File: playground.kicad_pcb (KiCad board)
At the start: 2 copper layers, 80 x 80 mm, 75 parts, among them IC1 TXU0101DBVR, IC11 LM3940IMP-3.3_NOPB, IC2 TXU0101DBVR, IC3 TXU0101DBVR, IC4 TXU0101DBVR, IC5 TXU0101DBVR, IC6 TXU0101DBVR, IC7 TXU0101DBVR, IC8 TXU0101DBVR, IC9 L293DD, J1 67643-2910, J2 Pump, J3 Fan, J4 Valve, J5 Conn_02x05_Counter_Clockwise, J6 MOLEX POWER CONNECTOR, SW1 SW_DIP_x01, U2 ATSAMD21G18A-A, Y1 32.768kHz

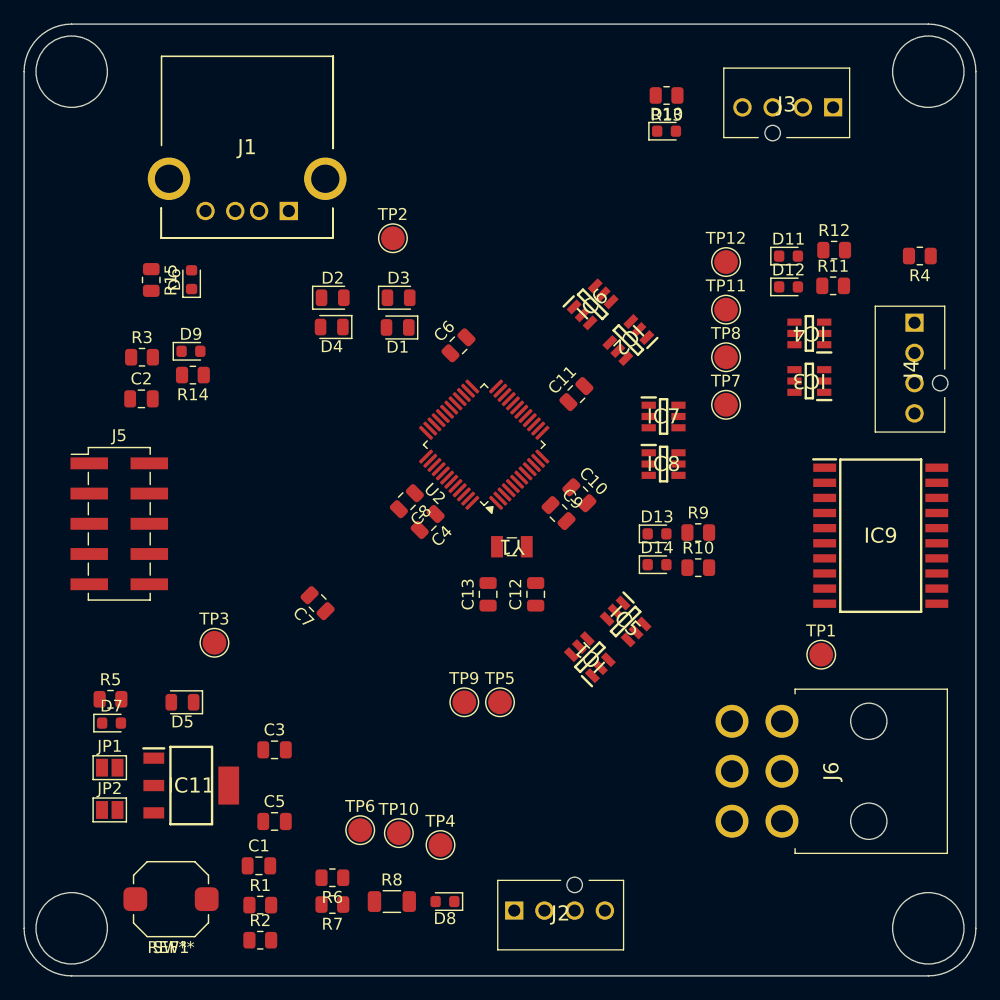
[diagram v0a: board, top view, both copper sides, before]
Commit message: Updated layout and schem
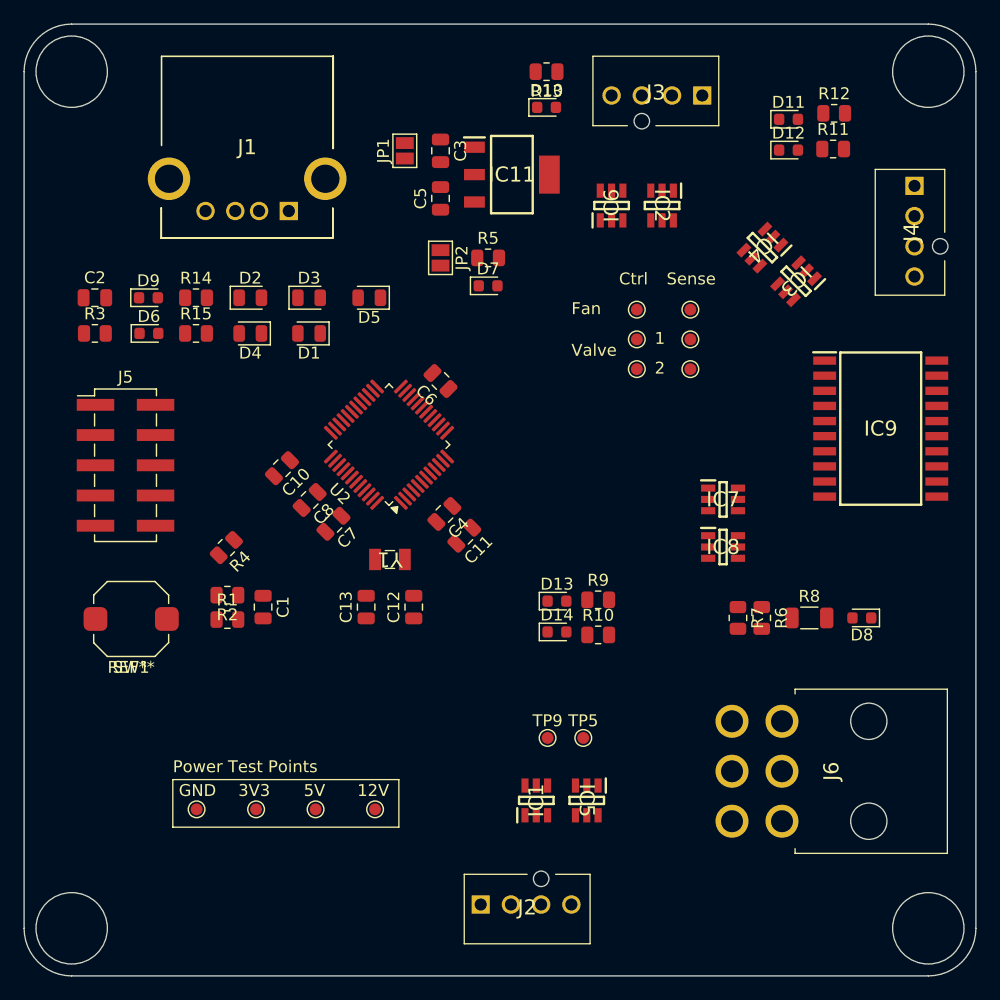
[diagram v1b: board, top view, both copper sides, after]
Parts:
- removed C9: 1u, Capacitor_SMD:C_0805_2012Metric
- TP1, TP10, TP11, TP12, TP2, TP3, TP4, TP5, TP6, TP7, TP8, TP9: footprint TestPoint:TestPoint_Pad_D2.0mm -> TestPoint:TestPoint_Pad_D1.0mm
- moved R4 63.2 mm to (67.0, 94.0), turned to -135 degrees
- moved IC11 58.0 mm to (91.0, 62.6)
- moved JP1 57.5 mm to (82.0, 60.6), turned to 90 degrees
- moved C5 54.2 mm to (85.0, 64.6), turned to 90 degrees
- moved JP2 54.1 mm to (85.0, 69.6), turned to -90 degrees
- moved C3 52.2 mm to (85.0, 60.6), turned to -90 degrees
- moved TP10 50.4 mm to (106.0, 74.0)
- moved TP6 49.5 mm to (101.5, 74.0)
- moved R5 48.8 mm to (89.0, 69.6)
- moved D7 48.5 mm to (89.0, 72.0)
- moved TP2 48.4 mm to (74.5, 116.0)
- moved R8 42.4 mm to (116.0, 99.9)
- moved D8 42.4 mm to (120.4, 99.9)
- moved R6 42.2 mm to (112.0, 99.9), turned to -90 degrees
- moved R7 41.7 mm to (110.0, 99.9), turned to -90 degrees
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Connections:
- net Net-(R6-Pad1) renamed /LEDs/12v_PWD_LED_VOL_DIV
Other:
- board text added: "1"
- board text added: "12V"
- board text added: "2"
- board text added: "3V3"
- board text added: "5V"
- board text added: "Ctrl"
- board text added: "Fan"
- board text added: "GND"
- board text added: "Power Test Points"
- board text added: "Sense"
- board text added: "Valve"
